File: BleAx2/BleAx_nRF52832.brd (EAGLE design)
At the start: 32.8 x 20.1 mm, 44 parts, among them CN1 6p-2.54, J1 2.0MM-90D, Q2 32MHz, U1 NRF52832, U2 MCP73832T-2ACI/OT-SOT23-5, U4 MIC5225-3.3, X2 32.768kHz

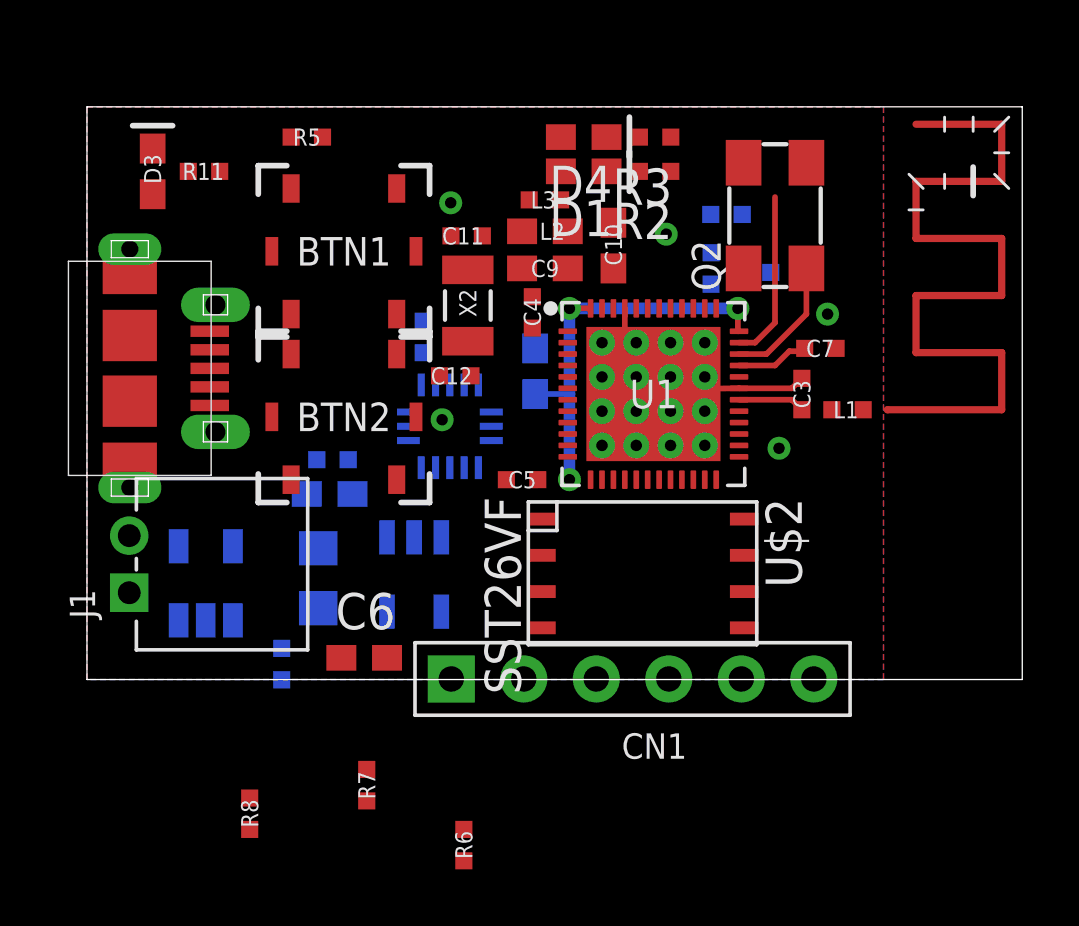
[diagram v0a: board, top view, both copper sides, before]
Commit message: evolve
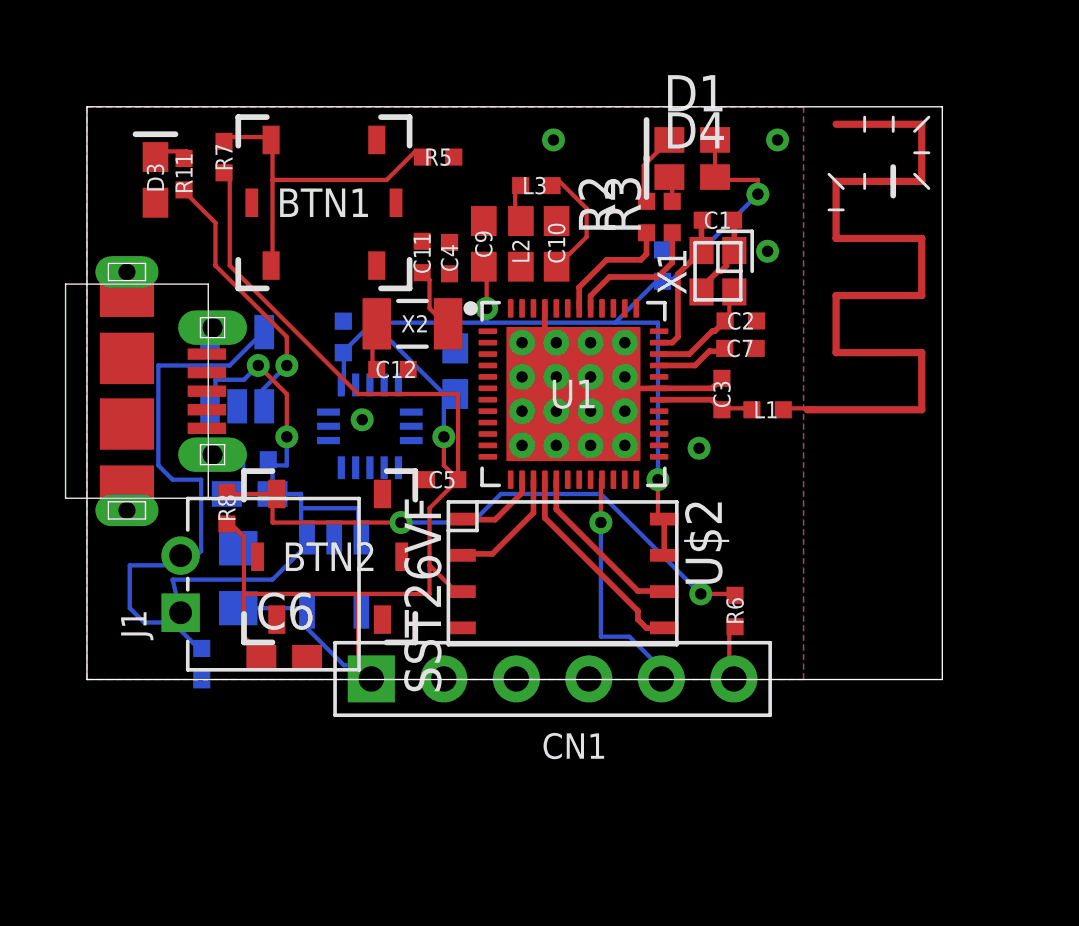
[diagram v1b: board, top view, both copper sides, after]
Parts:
- removed Q2: 32MHz, crystal-geyer_V1_0:5.0X3.2_KX-9A
- added X1: FA-128, crystals:FA-128
- C1, C2: value 12pF -> 10pF
- moved R7 22.6 mm to (4.80, 18.3)
- moved R6 12.5 mm to (22.7, 2.40)
- moved R8 10.7 mm to (4.90, 6.00)
- moved U2 7.58 mm to (5.26, 10.9)
- moved BTN2 4.93 mm to (8.50, 4.30)
- moved R5 4.65 mm to (12.3, 18.3)
- moved D4 4.05 mm to (21.2, 17.6), turned to 0 degrees
- moved D1 3.96 mm to (21.2, 18.9), turned to 0 degrees
- moved C4 3.47 mm to (12.7, 14.8)
- moved R3 2.86 mm to (20.5, 16.2), turned to 90 degrees
- moved ANT1 2.80 mm to (25.2, 9.45)
- moved C3 2.80 mm to (22.2, 10.0)
- moved C5 2.80 mm to (12.4, 7.00)
- moved C6 2.80 mm to (6.91, 0.76)
- moved C7 2.80 mm to (22.9, 11.6)
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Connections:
- net GND: now also X1.2, X1.4
- net MISO_02: now also U1.15; no longer U1.14
- net N$3: now also X1.3; no longer Q2.3
- net SST26_CE: now also U1.14; no longer U1.15
- net X1: now also X1.1; no longer Q2.1
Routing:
- net VDD_P3V3: track 14.7 -> 84.0 mm, vias 3 -> 4
- net N$6: track 0.00 -> 20.8 mm, vias 0 -> 2
- net VDD_BATT: track 0.00 -> 20.8 mm, vias 0 -> 2
- net N$1: track 0.00 -> 19.3 mm
- net N$7: track 0.00 -> 12.0 mm
- net N$10: track 0.00 -> 9.52 mm, vias 0 -> 1
- net P0.18/SWO: track 0.00 -> 8.45 mm, vias 0 -> 1
- net MOSI_02: track 0.00 -> 7.30 mm
- net SCK_02: track 0.00 -> 6.01 mm
- net LED_02: track 0.00 -> 4.83 mm
- net LED_01: track 0.00 -> 4.33 mm
- net MISO_02: track 0.00 -> 4.30 mm
- net DEC4: track 0.00 -> 4.18 mm
- net GND: track 23.9 -> 27.0 mm
- net SST26_CE: track 0.00 -> 2.98 mm
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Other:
- board size 32.8 x 20.1 mm -> 30 x 20.1 mm
